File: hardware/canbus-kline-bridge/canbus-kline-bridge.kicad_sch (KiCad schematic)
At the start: 36 parts, among them J1 USB_B_Micro, J2 SWD, J4 CANBus, J5 CANBus, J6 K-Line, Q1 2N7002, Q2 2N7002, U1 MCP1754S-3302xCB, U2 STM32F042F6Px, U3 Voltage Regulator, U4 MCP2562HD, U5 MC33660BEFR2

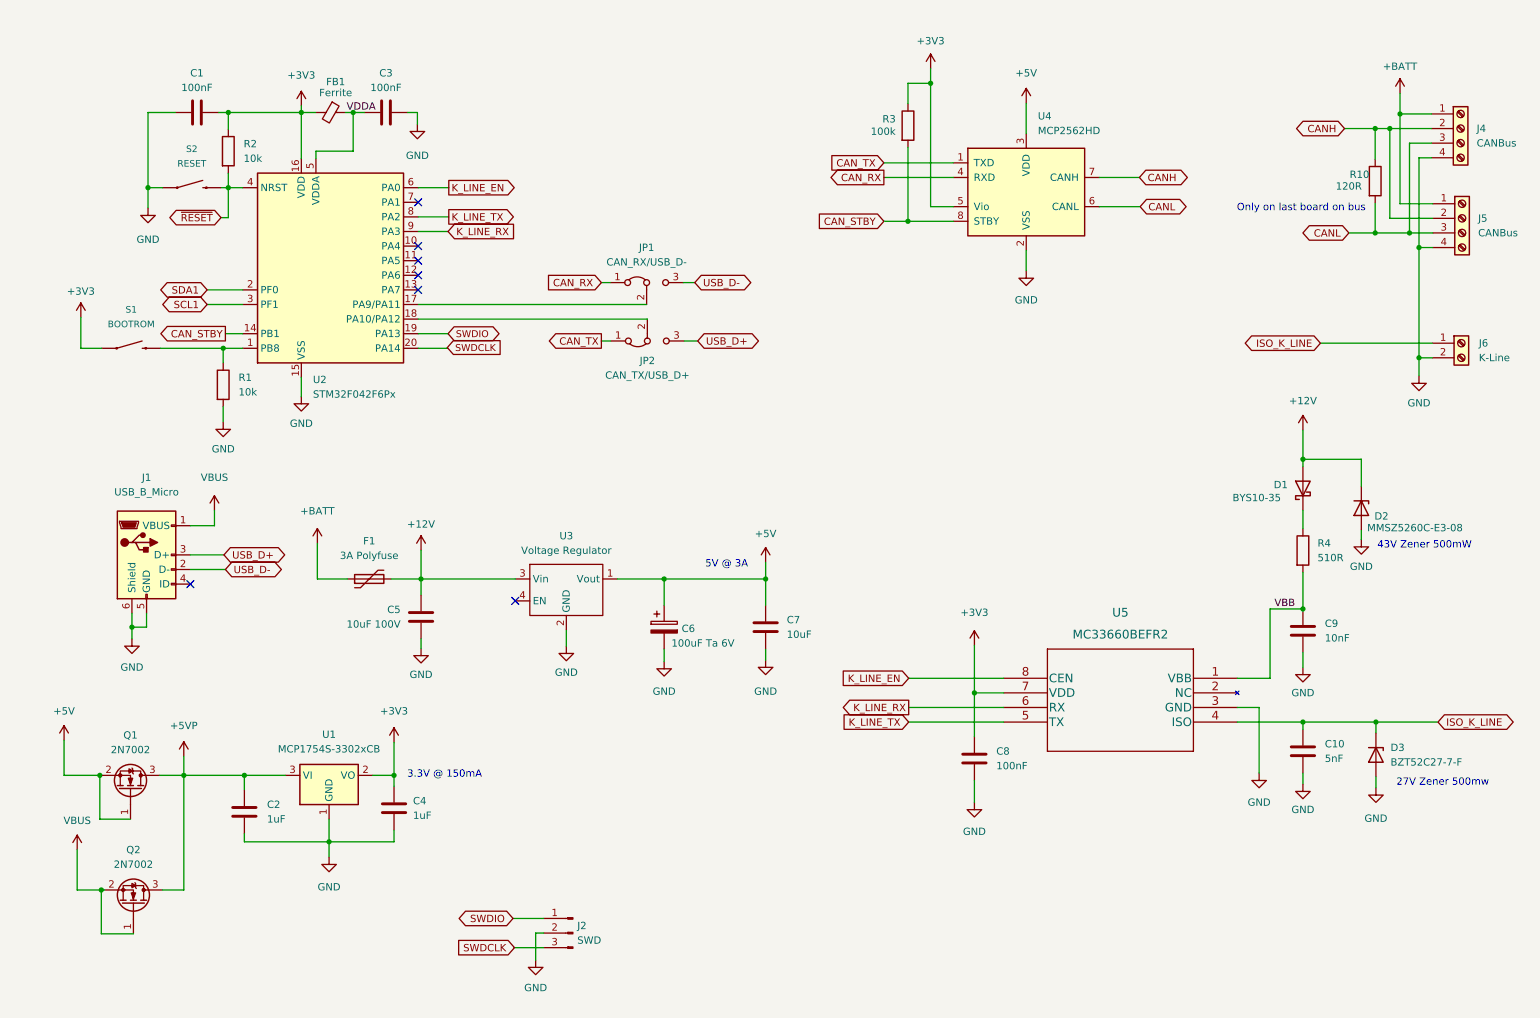
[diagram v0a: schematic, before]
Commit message: Working on the kline bridge a bit more
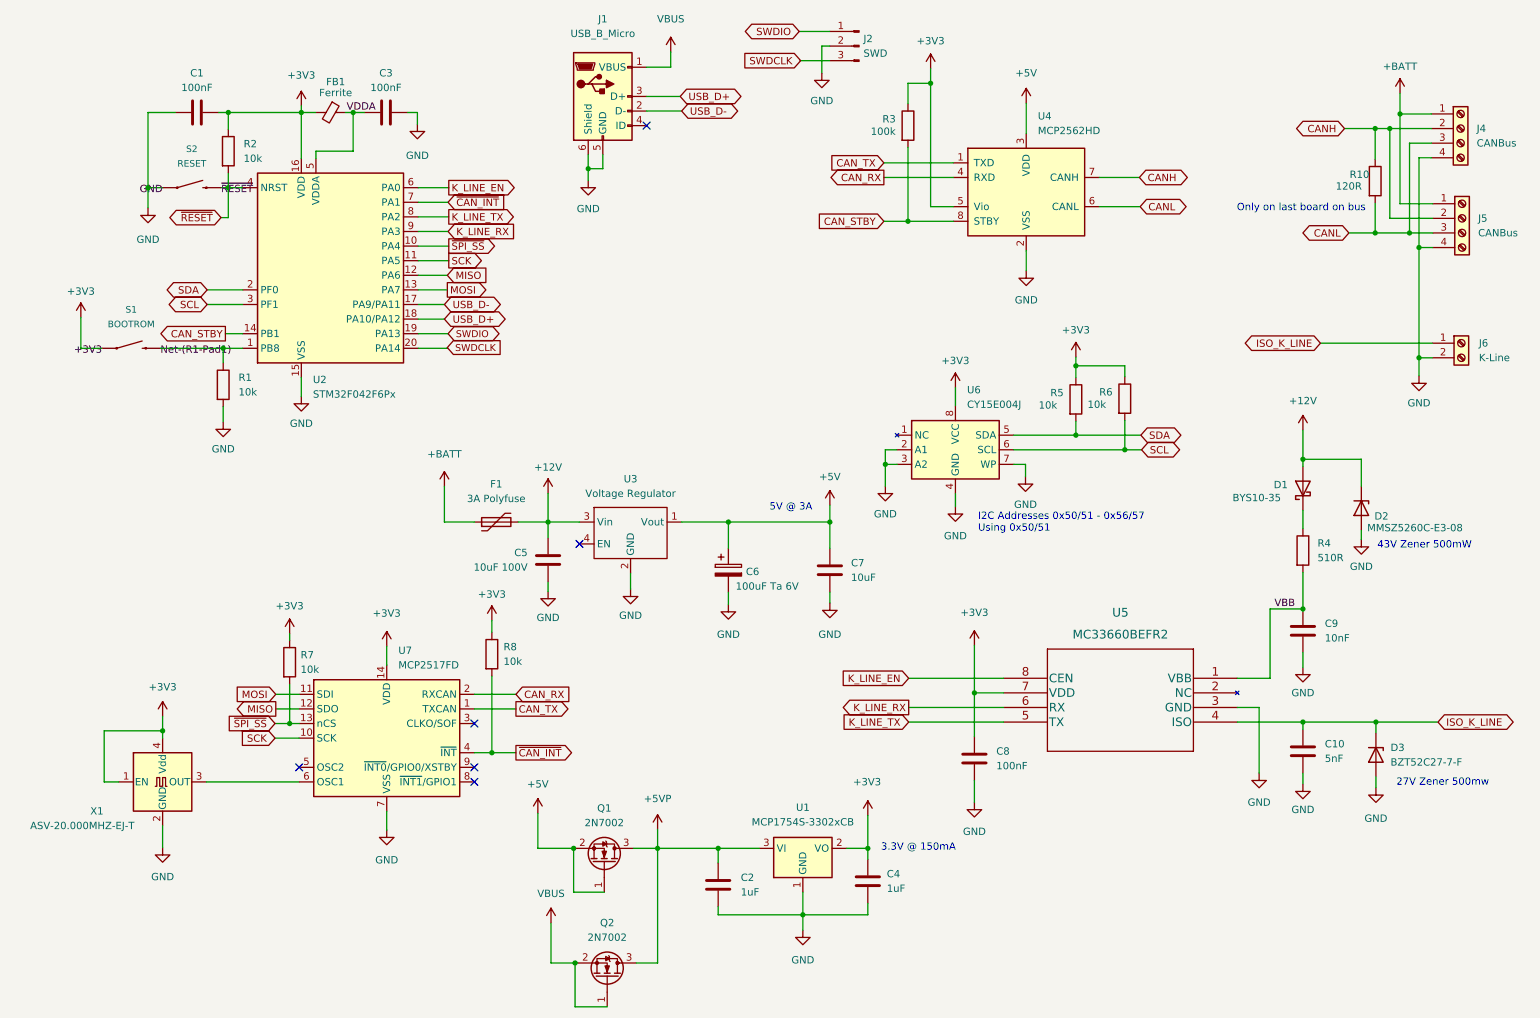
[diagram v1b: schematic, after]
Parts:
- removed JP1: CAN_RX/USB_D-, Connector_PinHeader_2.54mm:PinHeader_1x03_P2.54mm_Vertical, symbol Jumper:Jumper_3_Bridged12
- removed JP2: CAN_TX/USB_D+, Connector_PinHeader_2.54mm:PinHeader_1x03_P2.54mm_Vertical, symbol Jumper:Jumper_3_Bridged12
- added R5, R6, R7, R8: 10k, Resistor_SMD:R_0805_2012Metric_Pad1.20x1.40mm_HandSolder, symbol Device:R
- added U6: CY15E004J, Package_SO:SOIC-8_5.23x5.23mm_P1.27mm, symbol Beirdo:CY15E004J
- added U7: MCP2517FD, Package_SO:SOIC-14_3.9x8.7mm_P1.27mm, symbol Interface_CAN_LIN:MCP2517FD-xSL
- added X1: ASV-20.000MHZ-EJ-T, Oscillator:Oscillator_SMD_Abracon_ASV-4Pin_7.0x5.1mm, symbol Oscillator:ASV-xxxMHz
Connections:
- net +3V3: now also S1.2 (1), R5.1, R6.1, R7.1, R8.1, U6.8 (VCC), U7.14 (VDD), X1.1 (EN), X1.4 (Vdd)
- net CAN_RX: now also U7.2 (RXCAN)
- net CAN_TX: now also U7.1 (TXCAN)
- net GND: now also S2.2 (1), U6.2 (A1), U6.3 (A2), U6.4 (GND), U6.7 (WP), U7.7 (VSS), X1.2 (GND)
- net USB_D+: now also U2.18 (PA10/PA12)
- net USB_D-: now also U2.17 (PA9/PA11)
- net ~{RESET}: now also S2.4 (2)
- net Net-(R1-Pad1): now reaches S1.4 (2)
- net ~{SPI_SS}: now reaches U2.10 (PA4)
- net ~{SPI_SS}: now also R7.2, U7.13 (nCS)
- net SCK: now reaches U2.11 (PA5)
- net SCK: now also U7.10 (SCK)
- net MISO: now reaches U2.12 (PA6)
- net MISO: now also U7.12 (SDO)
- net MOSI: now reaches U2.13 (PA7)
- net MOSI: now also U7.11 (SDI)
- net ~{CAN_INT}: now reaches U2.7 (PA1)
- net ~{CAN_INT}: now also R8.2, U7.4 (~{INT})
- net SCL1 renamed SCL
- net SCL: now also R6.2, U6.6 (SCL)
- net SDA1 renamed SDA
- net SDA: now also R5.2, U6.5 (SDA)
- new net: U7.6 (OSC1), X1.3 (OUT)
- no-connect marks 7 -> 6
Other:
- note added: "I2C Addresses 0x50/51 - 0x56/57 Using 0x50/51"
- moved on the sheet: C2, C4, C5, C6, C7, F1, J1, J2, Q1, Q2, U1, U3
